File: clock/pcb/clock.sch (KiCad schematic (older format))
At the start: 41 parts, among them CON1 AVR-ISP-6, IC1 ATTINY44A-SS, P1 USB_OTG, Q1 Q_NMOS_DGS, Q10 Q_NMOS_DGS, Q11 Q_PMOS_DGS, Q12 Q_NPN_BCE, Q13 Q_NPN_BCE, Q2 Q_NPN_BCE, Q3 Q_NPN_BCE, Q4 Q_NMOS_DGS, Q5 Q_PMOS_DGS, Q6 Q_NMOS_DGS, Q7 Q_PMOS_DGS, Q8 Q_NMOS_DGS, Q9 Q_PMOS_DGS

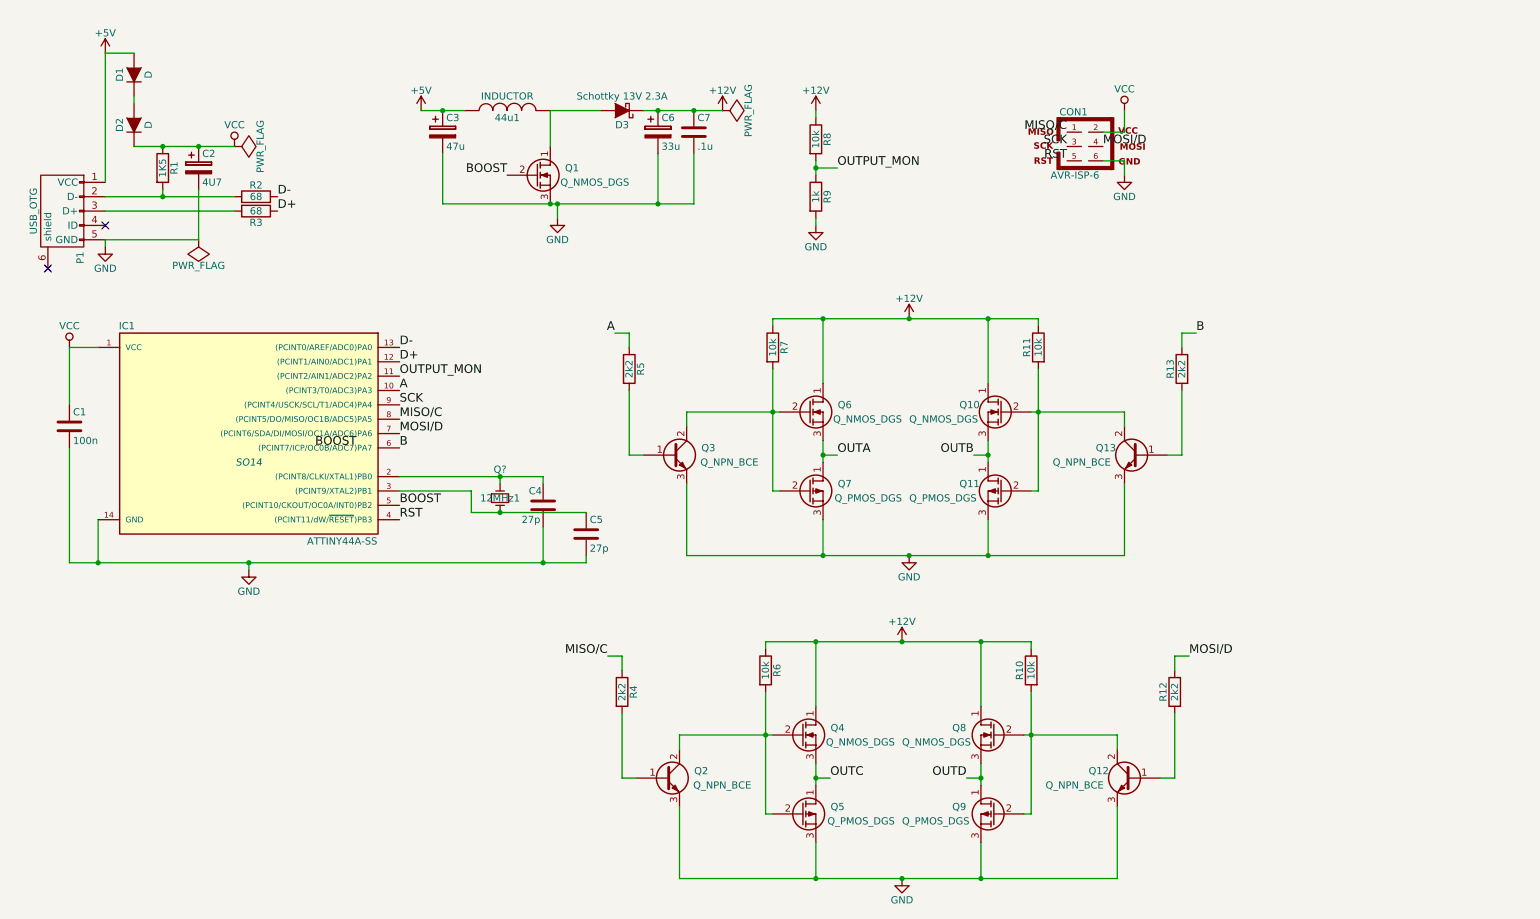
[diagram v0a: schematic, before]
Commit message: stm
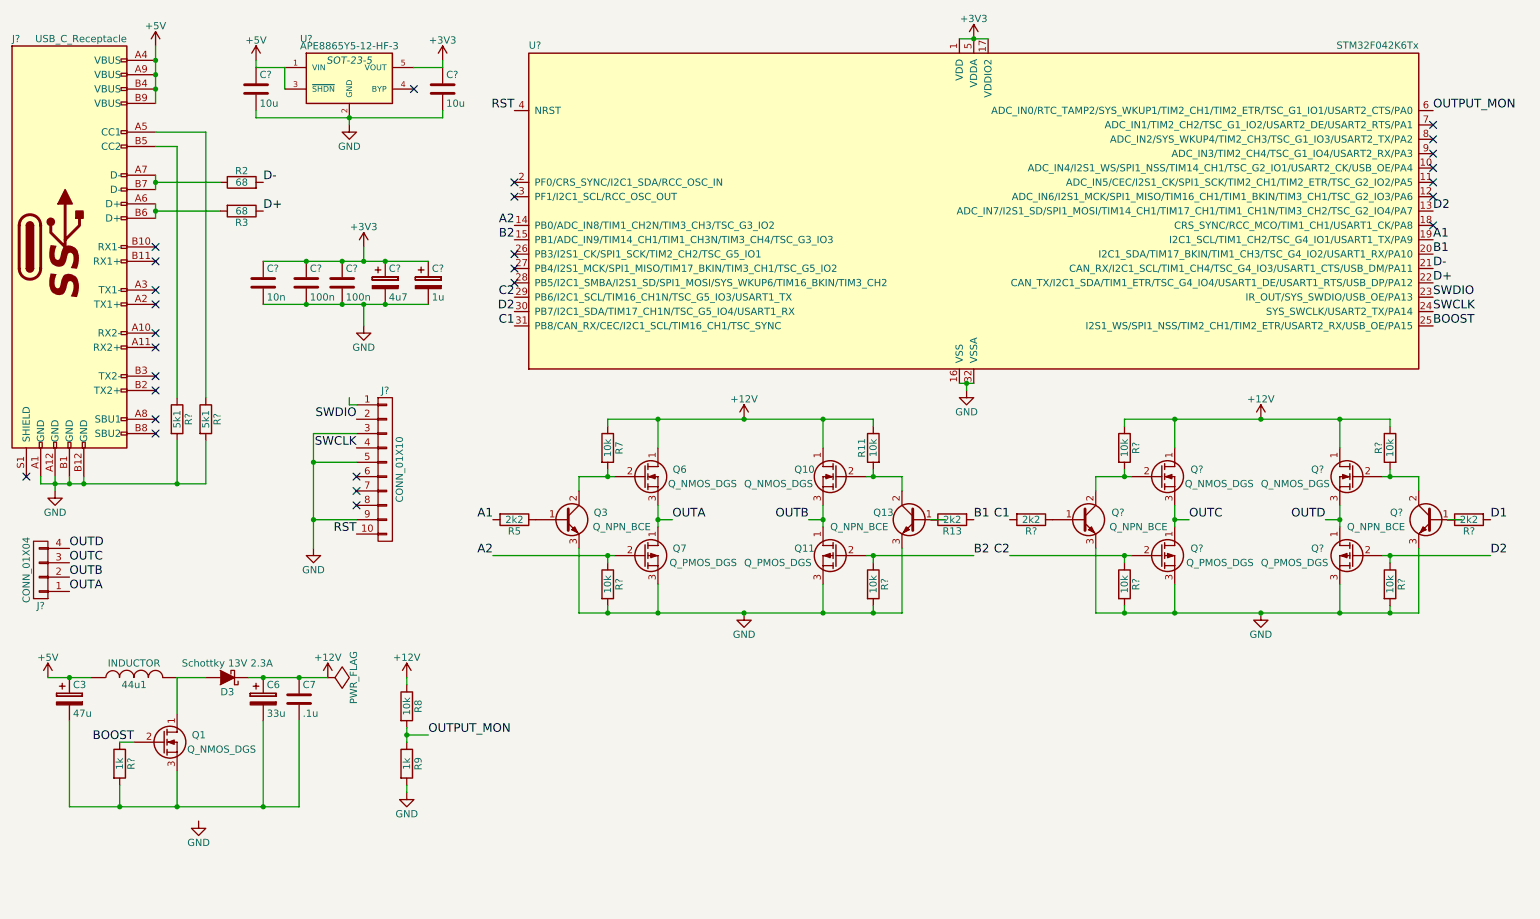
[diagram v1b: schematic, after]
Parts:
- removed 12MHz1: Q?, symbol Crystal_Small
- removed C1: 100n, symbol C
- removed C2: 4U7, symbol CP
- removed C4, C5: 27p, symbol C
- removed CON1: AVR-ISP-6, AVR-ISP-6, symbol AVR-ISP-6
- removed D1, D2: D, symbol D
- removed IC1: ATTINY44A-SS, SO14, symbol ATTINY44A-SS
- removed P1: USB_OTG, symbol USB_OTG
- removed Q12, Q2: Q_NPN_BCE, symbol Q_NPN_BCE
- removed Q4, Q8: Q_NMOS_DGS, symbol Q_NMOS_DGS
- removed Q5, Q9: Q_PMOS_DGS, symbol Q_PMOS_DGS
- removed R1: 1K5, symbol R
- removed R10, R6: 10k, symbol R
- removed R12, R4: 2k2, symbol R
- added C? (x2): 100n, symbol C
- added C?: 4u7, symbol CP
- added C?: 1u, symbol CP
- added C?: 10n, symbol C
- added C? (x2): 10u, symbol C
- added J?: USB_C_Receptacle, symbol USB_C_Receptacle
- added J?: CONN_01X04, symbol CONN_01X04
- added J?: CONN_01X10, symbol CONN_01X10
- added Q? (x2): Q_PMOS_DGS, symbol Q_PMOS_DGS
- added Q? (x2): Q_NMOS_DGS, symbol Q_NMOS_DGS
- added Q? (x2): Q_NPN_BCE, symbol Q_NPN_BCE
- added R?: 1k, symbol R
- added R? (x6): 10k, symbol R
- added R? (x2): 5k1, symbol R
- added R? (x2): 2k2, symbol R
- added U?: STM32F042K6Tx, LQFP32, symbol STM32F042K6Tx
- added U?: APE8865Y5-12-HF-3, SOT-23-5, symbol APE8865Y5-12-HF-3
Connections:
- net A is gone; now on an unnamed net: R5.1
- net B is gone; now on an unnamed net: R13.1
- net +12V: now also Q?.1 (D), Q?.1 (D), R?.1, R?.1
- net +5V: now also C?.1, J?.A4 (VBUS), J?.A9 (VBUS), J?.B4 (VBUS), J?.B9 (VBUS), U?.1 (VIN), U?.3 (~SHDN~)
- net BOOST: now also R?.1, U?.25 (I2S1_WS/SPI1_NSS/TIM2_CH1/TIM2_ETR/USART2_RX/USB_OE/PA15)
- net D+: now also U?.22 (CAN_TX/I2C1_SDA/TIM1_ETR/TSC_G4_IO4/USART1_DE/USART1_RTS/USB_DP/PA12)
- net D-: now also U?.21 (CAN_RX/I2C1_SCL/TIM1_CH4/TSC_G4_IO3/USART1_CTS/USB_DM/PA11)
- net GND: now also C?.2, C?.2, C?.2, C?.2, C?.2, C?.2, C?.2, J?.3 (P3), J?.5 (P5), J?.9 (P9), J?.A1 (GND), J?.A12 (GND), J?.B1 (GND), J?.B12 (GND), Q?.3 (E), Q?.3 (E), Q?.3 (S), Q?.3 (S), R?.2, R?.2, R?.2, R?.2, R?.2, R?.2, U?.16 (VSS), U?.2 (GND), U?.32 (VSSA); no longer C3.2, C6.2, C7.2, Q1.3 (S)
- net OUTA: now also J?.1 (P1)
- net OUTB: now also J?.2 (P2)
- net OUTC: now also J?.3 (P3), Q?.1 (D), Q?.3 (S)
- net OUTD: now also J?.4 (P4), Q?.1 (D), Q?.3 (S)
- net OUTPUT_MON: now also U?.6 (ADC_IN0/RTC_TAMP2/SYS_WKUP1/TIM2_CH1/TIM2_ETR/TSC_G1_IO1/USART2_CTS/PA0)
- net RST: now also J?.10 (P10), U?.4 (NRST)
- net at R2.1: now also J?.A7 (D-), J?.B7 (D-)
- net at R3.2: now also J?.A6 (D+), J?.B6 (D+)
- net at Q3.2 (C), Q6.2 (G), R7.2: no longer Q7.2 (G)
- net at Q3.1 (B): no longer R5.2
- net at Q10.2 (G), Q13.2 (C), R11.2: no longer Q11.2 (G)
- net at Q13.1 (B): no longer R13.2
- new net: C3.2, C6.2, C7.2, Q1.3 (S), R?.2
- new net: J?.A5 (CC1), R?.1
- new net: J?.B5 (CC2), R?.1
- new net: Q?.2 (C), Q?.2 (G), R?.2 (x2)
- new net: Q?.1 (B), R?.1 (x2)
- new net +3V3: C?.1, C?.1, C?.1, C?.1, C?.1, C?.1, U?.1 (VDD), U?.17 (VDDIO2), U?.5 (VDDA), U?.5 (VOUT)
- new net A1: R5.2, U?.19 (I2C1_SCL/TIM1_CH2/TSC_G4_IO1/USART1_TX/PA9)
- new net A2: Q7.2 (G), R?.1, U?.14 (PB0/ADC_IN8/TIM1_CH2N/TIM3_CH3/TSC_G3_IO2)
- new net B1: R13.2, U?.20 (I2C1_SDA/TIM17_BKIN/TIM1_CH3/TSC_G4_IO2/USART1_RX/PA10)
- new net B2: Q11.2 (G), R?.1, U?.15 (PB1/ADC_IN9/TIM14_CH1/TIM1_CH3N/TIM3_CH4/TSC_G3_IO3)
- new net C1: R?.2, U?.31 (PB8/CAN_RX/CEC/I2C1_SCL/TIM16_CH1/TSC_SYNC)
- new net C2: Q?.2 (G), R?.1, U?.29 (PB6/I2C1_SCL/TIM16_CH1N/TSC_G5_IO3/USART1_TX)
- new net D1: R?.2
- new net D2: Q?.2 (G), R?.1, U?.13 (ADC_IN7/I2S1_SD/SPI1_MOSI/TIM14_CH1/TIM17_CH1/TIM1_CH1N/TIM3_CH2/TSC_G2_IO4/PA7), U?.30 (PB7/I2C1_SDA/TIM17_CH1N/TSC_G5_IO4/USART1_RX)
- new net SWCLK: J?.4 (P4), U?.24 (SYS_SWCLK/USART2_TX/PA14)
- new net SWDIO: J?.2 (P2), U?.23 (IR_OUT/SYS_SWDIO/USB_OE/PA13)
- no-connect marks 2 -> 27
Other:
- moved on the sheet: 44u1, C3, C6, C7, D3, Q1, Q10, Q11, Q13, Q3, Q6, Q7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
